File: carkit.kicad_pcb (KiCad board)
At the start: 2 copper layers, 100 x 45 mm, 55 parts, among them J1 Barrel_Jack, J2 Conn_01x02_Pin, J3 Conn_02x03_Odd_Even, J4 Conn_02x03_Odd_Even, J5 Conn_01x02_Pin, J6 Conn_01x02_Pin, P1 USB_C_Plug, SW1 SW_Push, SW2 SW_Push, U1 ESP32-C3-MINI-1, U2 LM2596SX-5.0/NOPB, U3 AMS1117-3.3, U4 DRV8876PWPR, U5 DRV8876PWPR

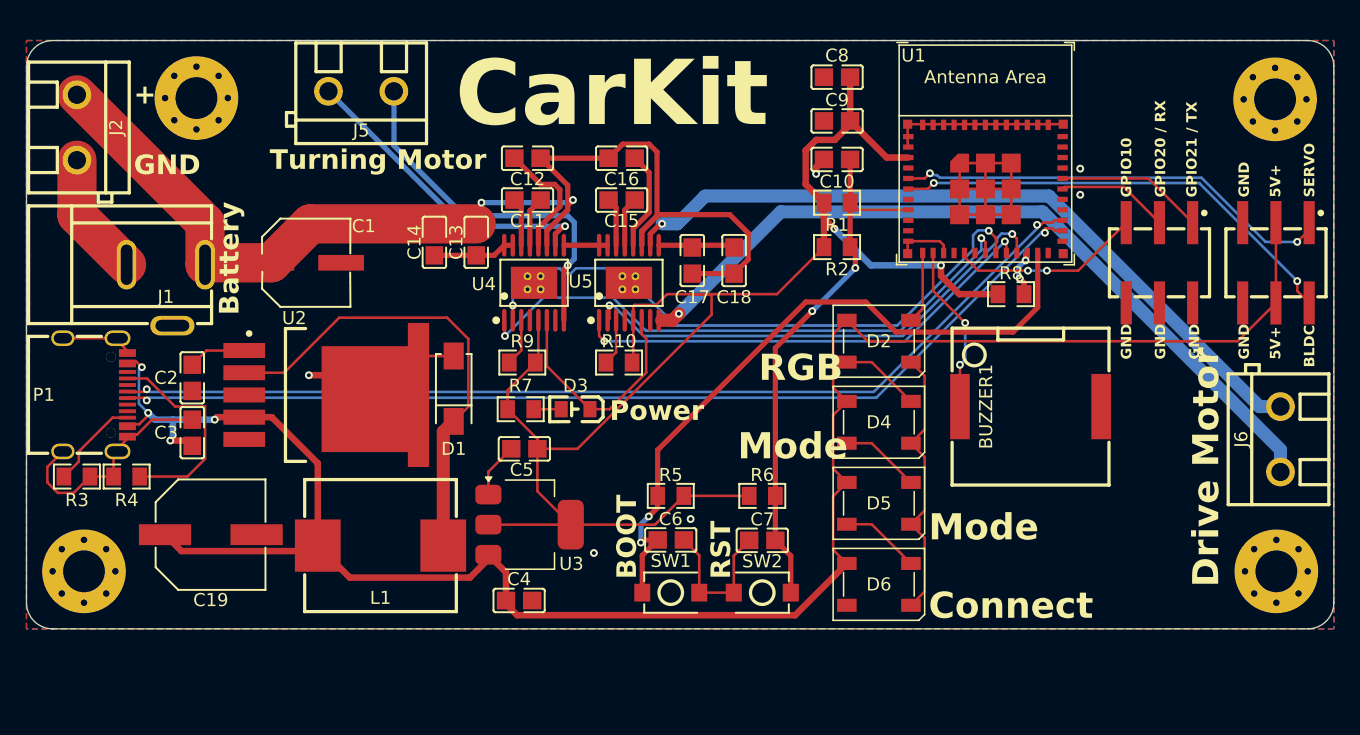
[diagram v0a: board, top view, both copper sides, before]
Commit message: Panelization Complete
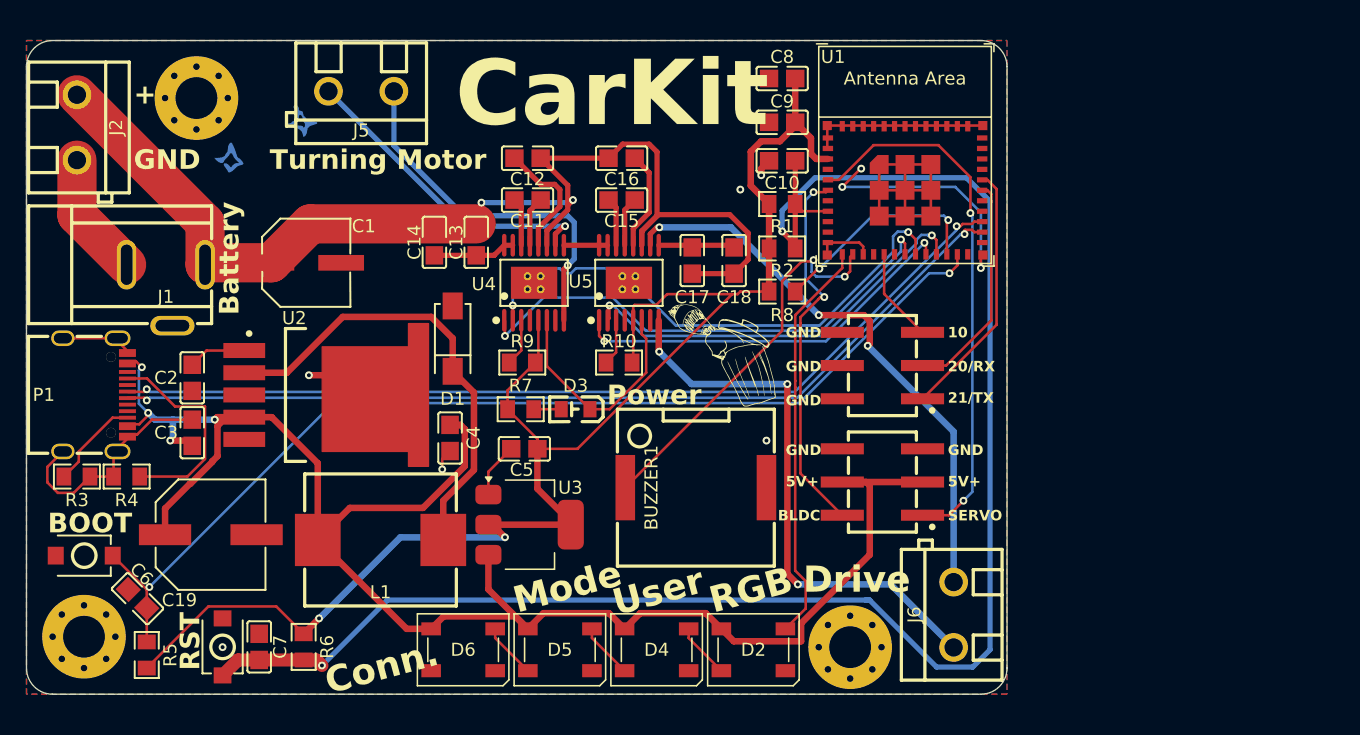
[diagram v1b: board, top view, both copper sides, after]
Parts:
- removed H4: MountingHole, MountingHole:MountingHole_3.2mm_M3_Pad_Via
- added G***: LOGO, LOGO, F.Cu at (67.8, 38.6)
- added G***: LOGO, LOGO, B.Cu at (45.9, 55.0)
- added G***: LOGO, LOGO, B.Cu at (79.2, 26.7)
- added G***: LOGO, LOGO, B.Cu at (52.7, 23.2)
- added G***: LOGO, LOGO, B.Cu at (39.2, 31.9)
- added G***: LOGO, LOGO, B.Cu at (69.5, 46.9)
- added G***: LOGO, LOGO, B.Cu at (65.2, 23.8)
- added G***: LOGO, LOGO, B.Cu at (28.8, 50.6)
- moved H3 53.0 mm to (77.4, 60.6)
- moved SW1 44.9 mm to (18.8, 53.6), turned to 180 degrees
- moved R5 41.9 mm to (23.6, 61.2), turned to 90 degrees
- moved SW2 41.5 mm to (29.4, 60.6), turned to 90 degrees
- moved C6 41.0 mm to (22.9, 56.9), turned to 180 degrees
- moved C7 39.3 mm to (32.2, 60.6), turned to 90 degrees
- moved R6 36.9 mm to (35.6, 60.6), turned to -90 degrees
- moved J3 32.6 mm to (80.0, 46.6), turned to 90 degrees
- moved D6 32.2 mm to (47.8, 60.8)
- moved J6 28.4 mm to (85.3, 58.1)
- moved D5 26.8 mm to (55.2, 60.8)
- moved BUZZER1 26.3 mm to (65.6, 48.4)
- moved D2 25.5 mm to (70.0, 60.8)
- moved D4 24.3 mm to (62.6, 60.8)
- moved J4 20.8 mm to (80.0, 37.7), turned to 90 degrees
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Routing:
- net CHIP_PU: track 41.0 -> 129.1 mm
- net GPIO 9: track 53.1 -> 80.8 mm
- net LED_DATA: track 5.52 -> 31.1 mm
- net GND: track 162.3 -> 142.5 mm, vias 6 -> 9
- net VCC_5V: track 153.6 -> 133.9 mm
- net M2+: track 60.0 -> 42.8 mm, vias 1 -> 3
- net BUZZER_DATA: track 12.9 -> 29.4 mm
- net M2-: track 56.9 -> 43.6 mm, vias 1 -> 3
- net GPIO 8: track 3.61 -> 16.9 mm
- net GPIO 20: track 8.60 -> 17.2 mm
- net GPIO 21: track 11.4 -> 19.8 mm
- net SERVO_PWM: track 33.9 -> 41.7 mm
- net GPIO 10: track 14.6 -> 7.18 mm, vias 2 -> 0
- net D-: track 77.3 -> 71.1 mm
- net D+: track 77.3 -> 71.1 mm
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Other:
- board size 100 x 45 mm -> 75 x 50 mm
- board text added: "10"
- board text added: "20/RX"
- board text added: "21/TX"
- board text added: "Conn."
- board text added: "Drive"
- board text added: "User"
- board text removed: "Connect"
- board text removed: "Drive Motor"
- board text removed: "GPIO10"
- board text removed: "GPIO20 / RX"
- board text removed: "GPIO21 / TX"
